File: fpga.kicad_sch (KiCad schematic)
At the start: 8 parts, among them J1 fpga_debug, U1 S25FL127S, U2 XC7A100T-FTG256

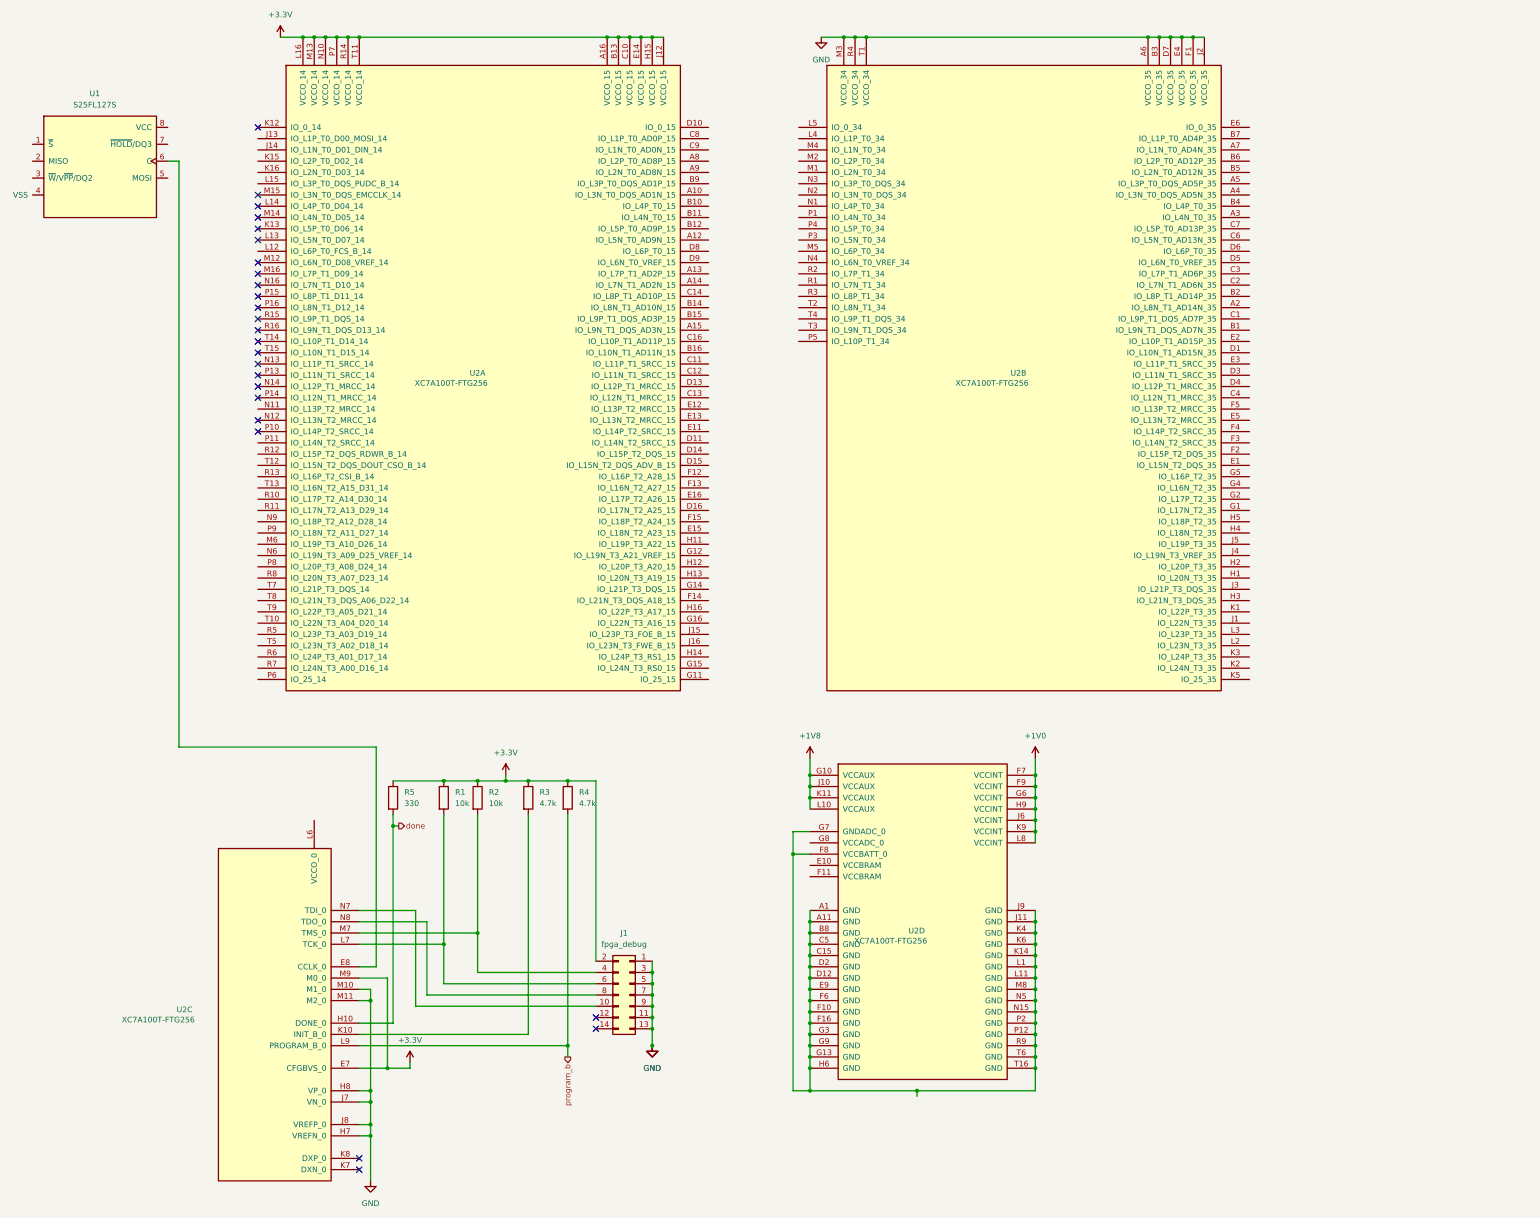
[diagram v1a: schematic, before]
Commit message: updates to fpga
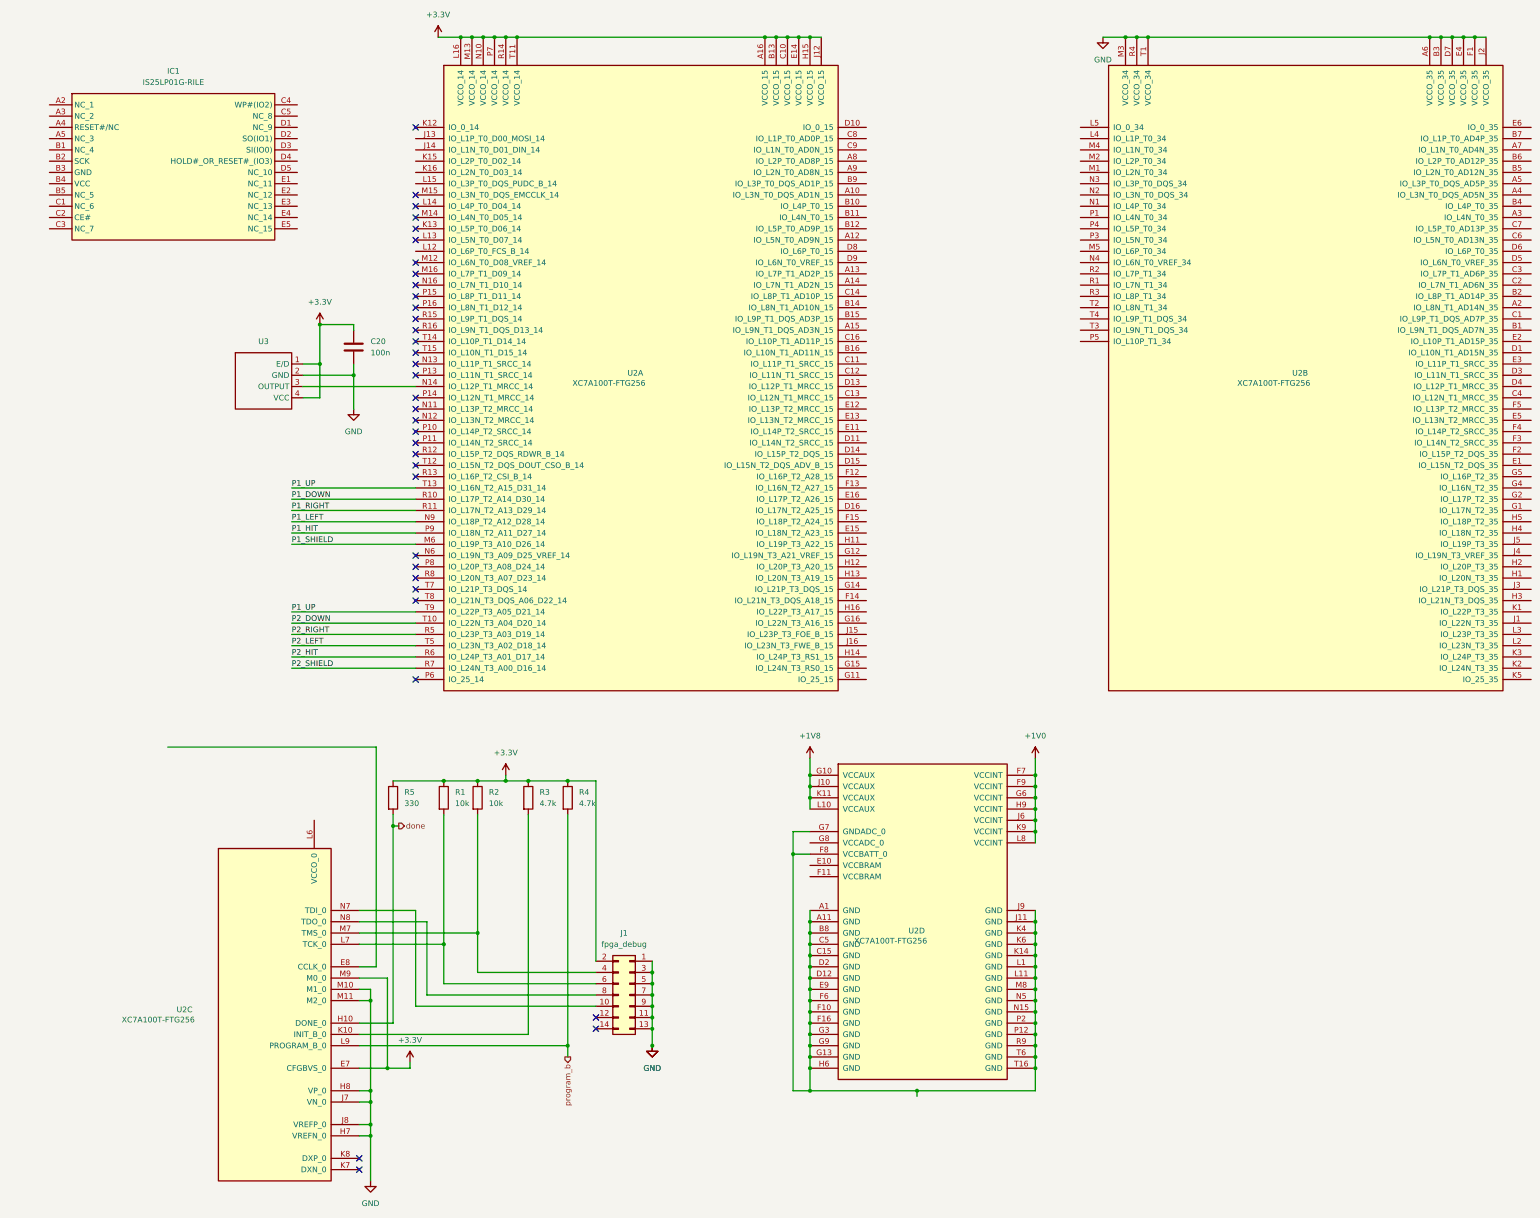
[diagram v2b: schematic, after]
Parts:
- removed U1: S25FL127S, Package_SO:SOIC-8_3.9x4.9mm_P1.27mm, symbol symbol_library:S25FL127S
- added C20: 100n, symbol Device:C
- added IC1: IS25LP01G-RILE, BGA24C100P5X5_600X800X140, symbol symbol_library:IS25LP01G-RILE
- added U3: (no value), Oscillator:Oscillator_DIP-14, symbol symbol_library:Oscillator
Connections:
- net +3.3V: now also C20.1, U3.1 (E/D), U3.4 (VCC)
- net GND: now also C20.2, U3.2 (GND)
- net P1_SHIELD: now reaches U2.M6 (IO_L19P_T3_A10_D26_14)
- net at U2.N14 (IO_L12P_T1_MRCC_14): now also U3.3 (OUTPUT)
- net P1_LEFT: now reaches U2.N9 (IO_L18P_T2_A12_D28_14)
- net P1_HIT: now reaches U2.P9 (IO_L18N_T2_A11_D27_14)
- net P1_DOWN: now reaches U2.R10 (IO_L17P_T2_A14_D30_14)
- net P1_RIGHT: now reaches U2.R11 (IO_L17N_T2_A13_D29_14)
- net P2_RIGHT: now reaches U2.R5 (IO_L23P_T3_A03_D19_14)
- net P2_HIT: now reaches U2.R6 (IO_L24P_T3_A01_D17_14)
- net P2_SHIELD: now reaches U2.R7 (IO_L24N_T3_A00_D16_14)
- net P2_DOWN: now reaches U2.T10 (IO_L22N_T3_A04_D20_14)
- net P1_UP: now reaches U2.T13 (IO_L16N_T2_A15_D31_14)
- net P1_UP: now also U2.T9 (IO_L22P_T3_A05_D21_14)
- net P2_LEFT: now reaches U2.T5 (IO_L23N_T3_A02_D18_14)
- no-connect marks 25 -> 35
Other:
- moved on the sheet: U2A, U2B
